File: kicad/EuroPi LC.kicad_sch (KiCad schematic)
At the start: 2 parts, among them U4 SEEEDUINO-XIAO

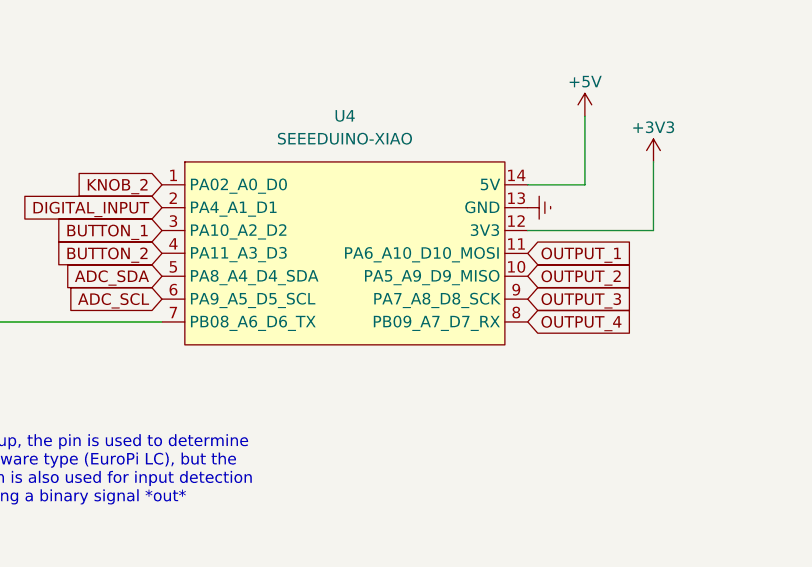
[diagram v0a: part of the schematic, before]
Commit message: reroute pcb
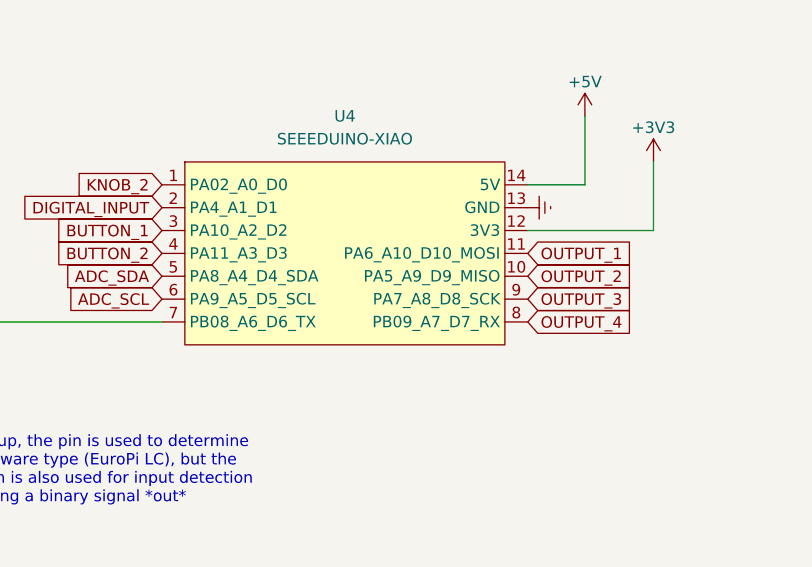
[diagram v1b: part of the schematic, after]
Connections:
- net BUTTON_2: now also U4.4 (PA11_A3_D3)
- net OUTPUT_4: now also U4.8 (PB09_A7_D7_RX)
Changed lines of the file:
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@@
     )
   )
-  (global_label "OUTPUT_4" (shape input) (at 107.9468 55.8649 0) (fields_autoplaced)
+  (global_label "OUTPUT_4" (shape input) (at 107.95 55.88 0) (fields_autoplaced)
     (effects (font (size 1.27 1.27)) (justify left))
-    (property "Intersheetrefs" "${INTERSHEET_REFS}" (at 120.2264 55.8649 0)
+    (property "Intersheetrefs" "${INTERSHEET_REFS}" (at 120.2296 55.88 0)
       (effects (font (size 1.27 1.27)) (justify left) hide)
     )
